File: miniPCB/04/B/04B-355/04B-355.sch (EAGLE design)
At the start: 45 parts

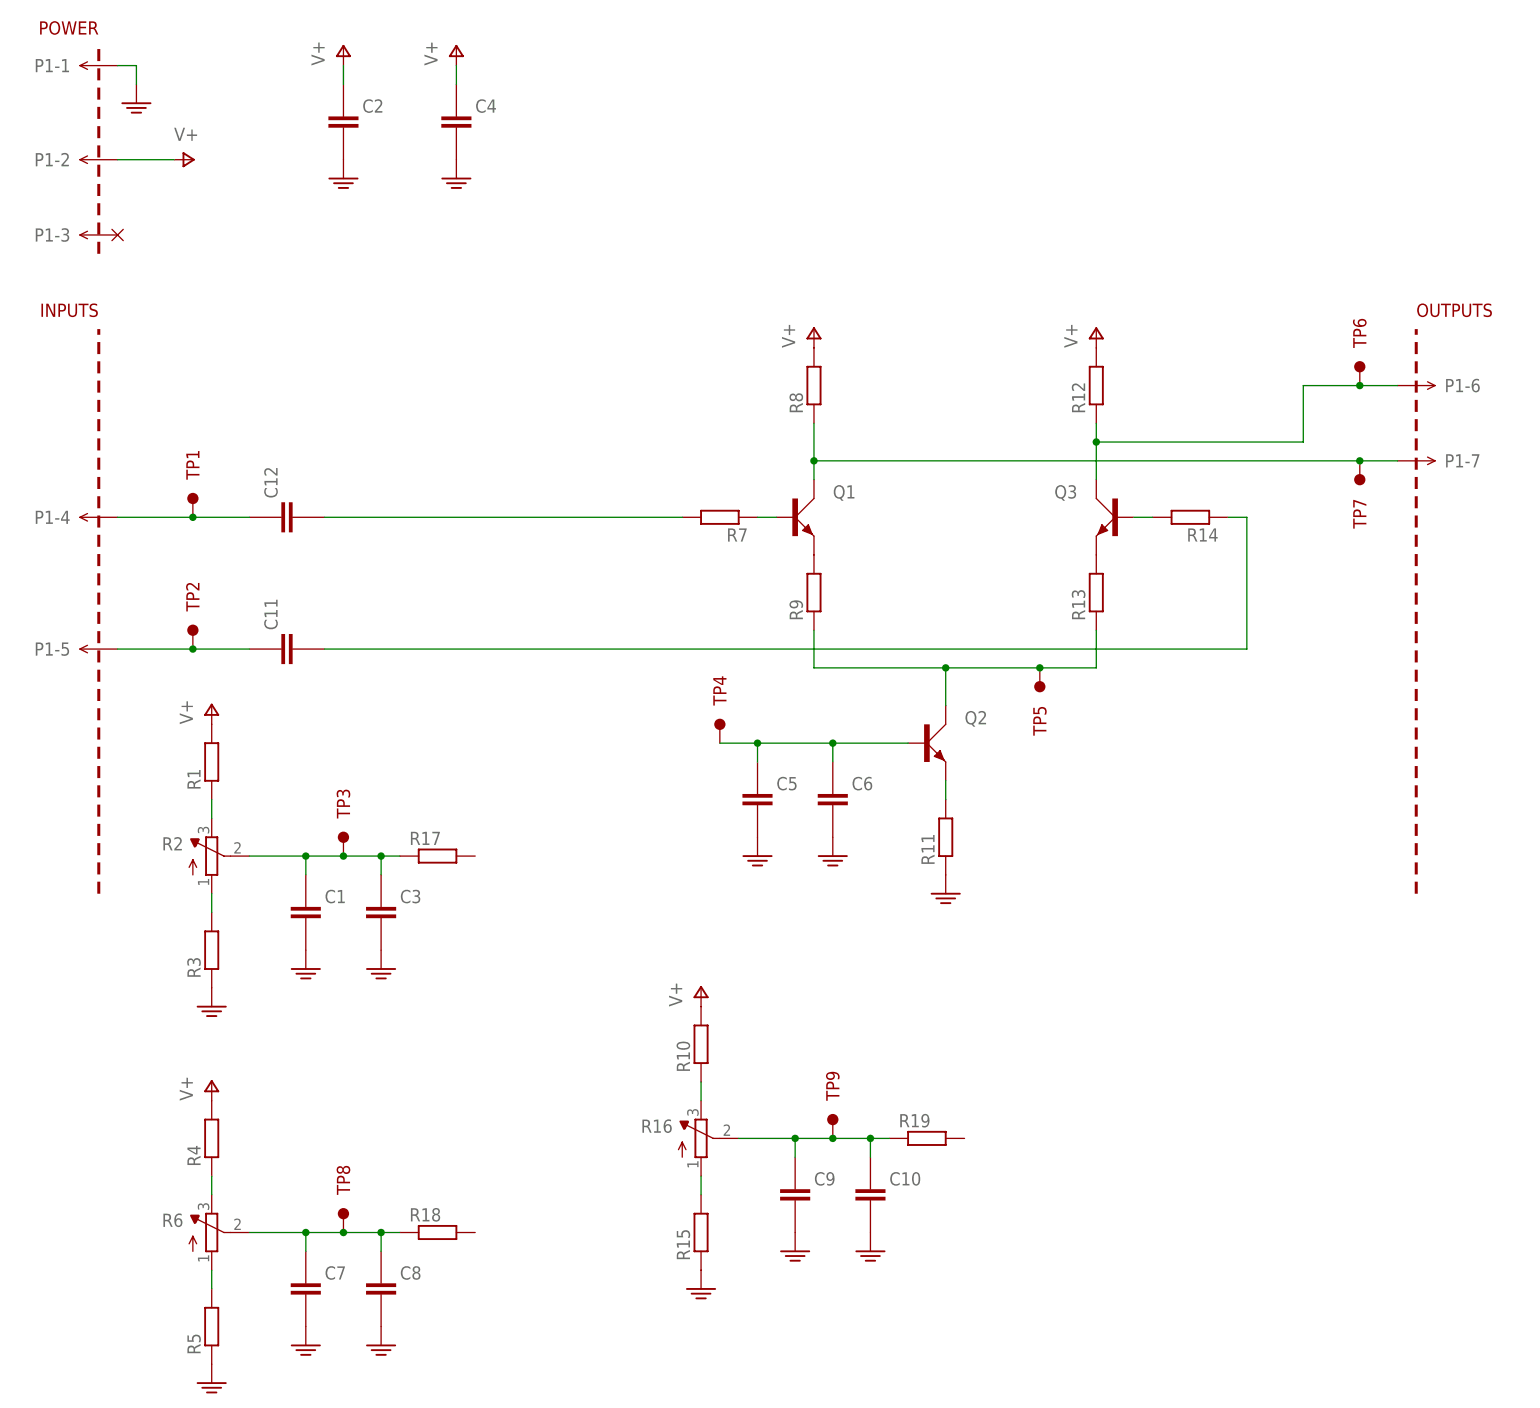
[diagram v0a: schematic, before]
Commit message: Attempting to fix my Git merge error.
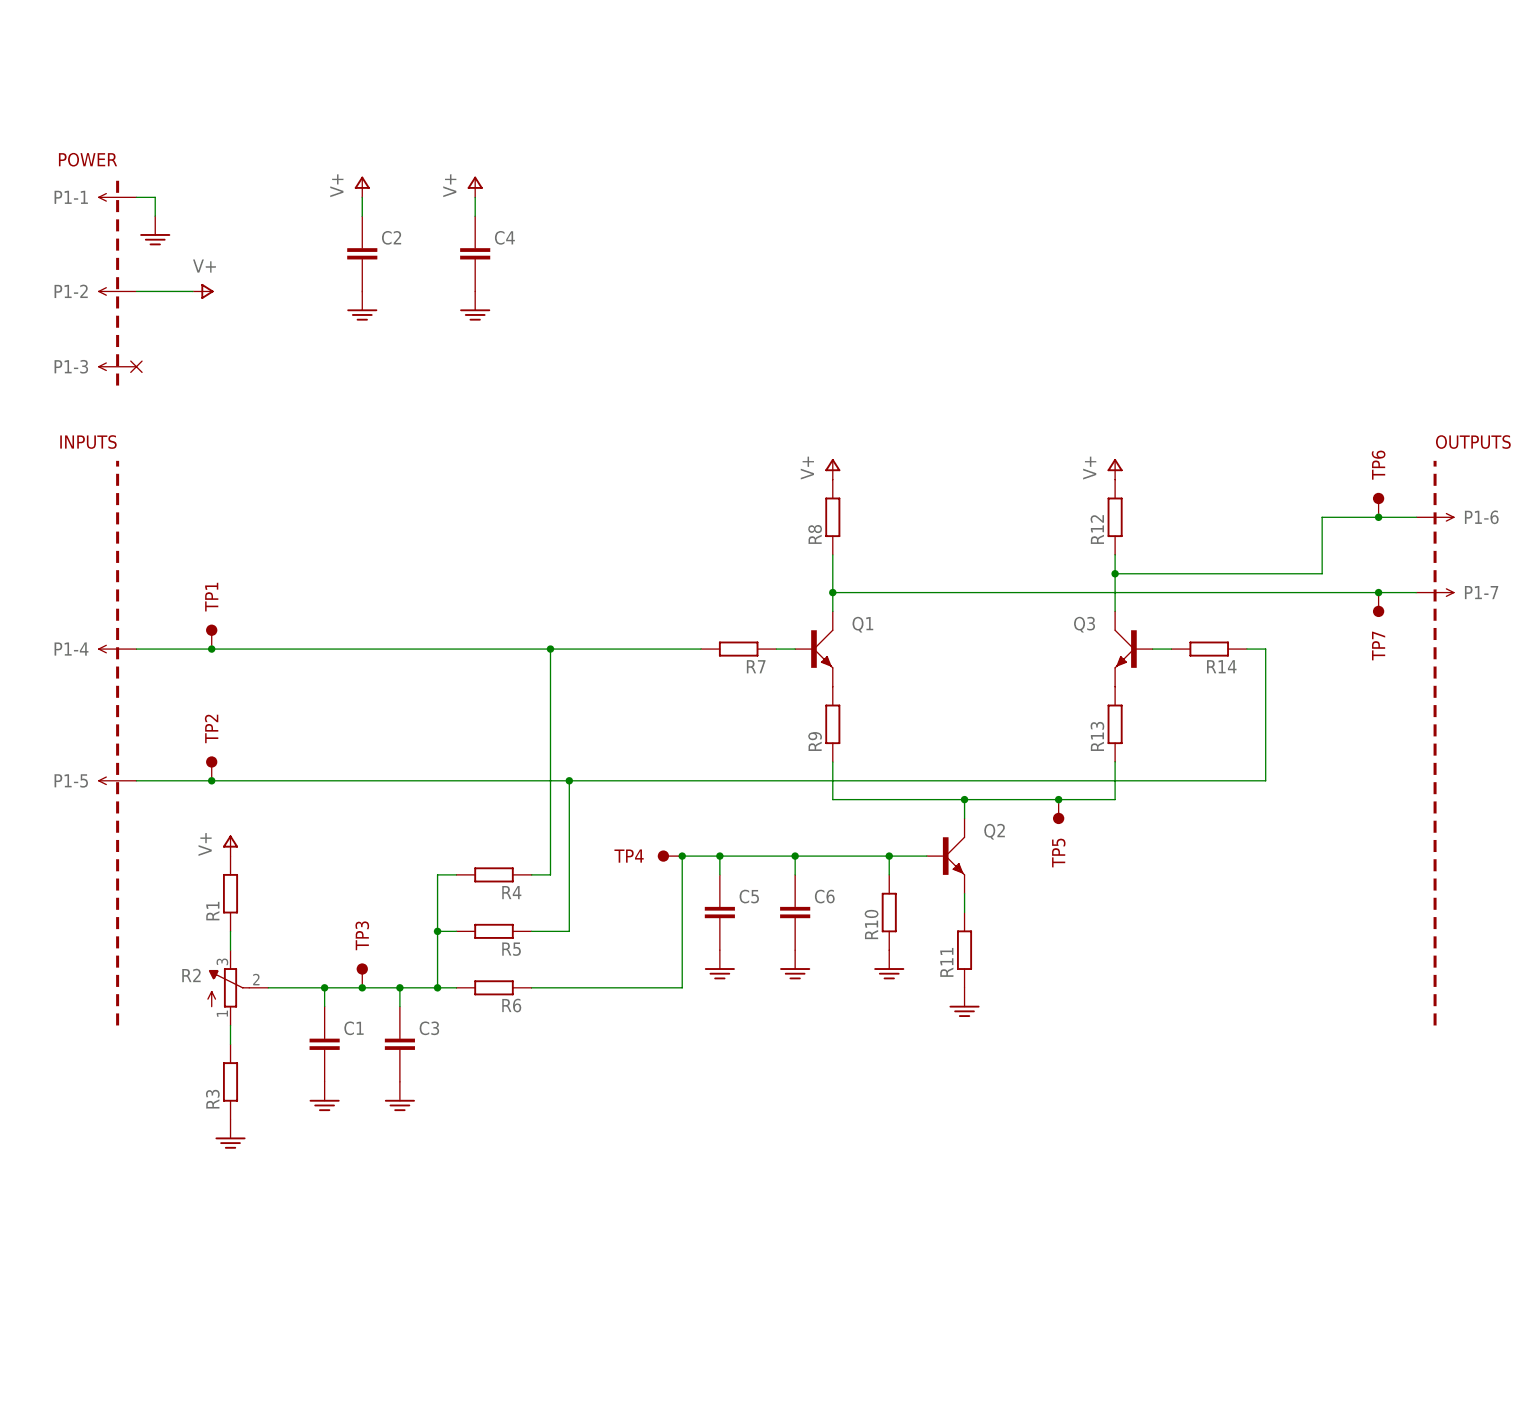
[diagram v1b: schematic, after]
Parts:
- removed C10, C8: (no value), minipcb:CAPACITOR_10
- removed C11, C12, C7, C9: (no value), minipcb:CAPACITORTHD
- removed R15, R17, R18, R19: (no value), minipcb:RESISTORTHD
- removed R16: (no value), minipcb:TRIMPOT0.100THD
- removed TP8, TP9: (no value), minipcb:TESTPOINTKE5000-SMTEXT
- R6: device minipcb:TRIMPOT0.100THD -> minipcb:RESISTORTHD
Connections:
- removed net N$15: R4.1, R6.E
- removed net N$16: R5.2, R6.A
- removed net N$17: C7.+, C8.+, R18.1, R6.S, TP8.1
- removed net N$18: R10.1, R16.E
- removed net N$19: R15.2, R16.A
- removed net N$20: C10.+, C9.+, R16.S, R19.1, TP9.1
- removed net N$21: C11.+, P1-5.1, TP2.1
- removed net N$22: C12.+, P1-4.1, TP1.1
- net GND: now also R10.1; no longer C10.-, C7.-, C8.-, C9.-, R15.1, R5.1
- net N$12: now also R10.2, R6.1
- net N$14: now also R4.2, R5.2, R6.2; no longer R17.1
- net N$8: now also P1-4.1, R4.1, TP1.1; no longer C12.-
- net N$9: now also P1-5.1, R5.1, TP2.1; no longer C11.-
- net V+: no longer R10.2, R4.2
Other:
- moved on the sheet: C1, C2, C3, C4, C5, C6, P1-1, P1-2, P1-3, P1-4, P1-5, P1-6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

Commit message: Attempting to fix my Git merge error.
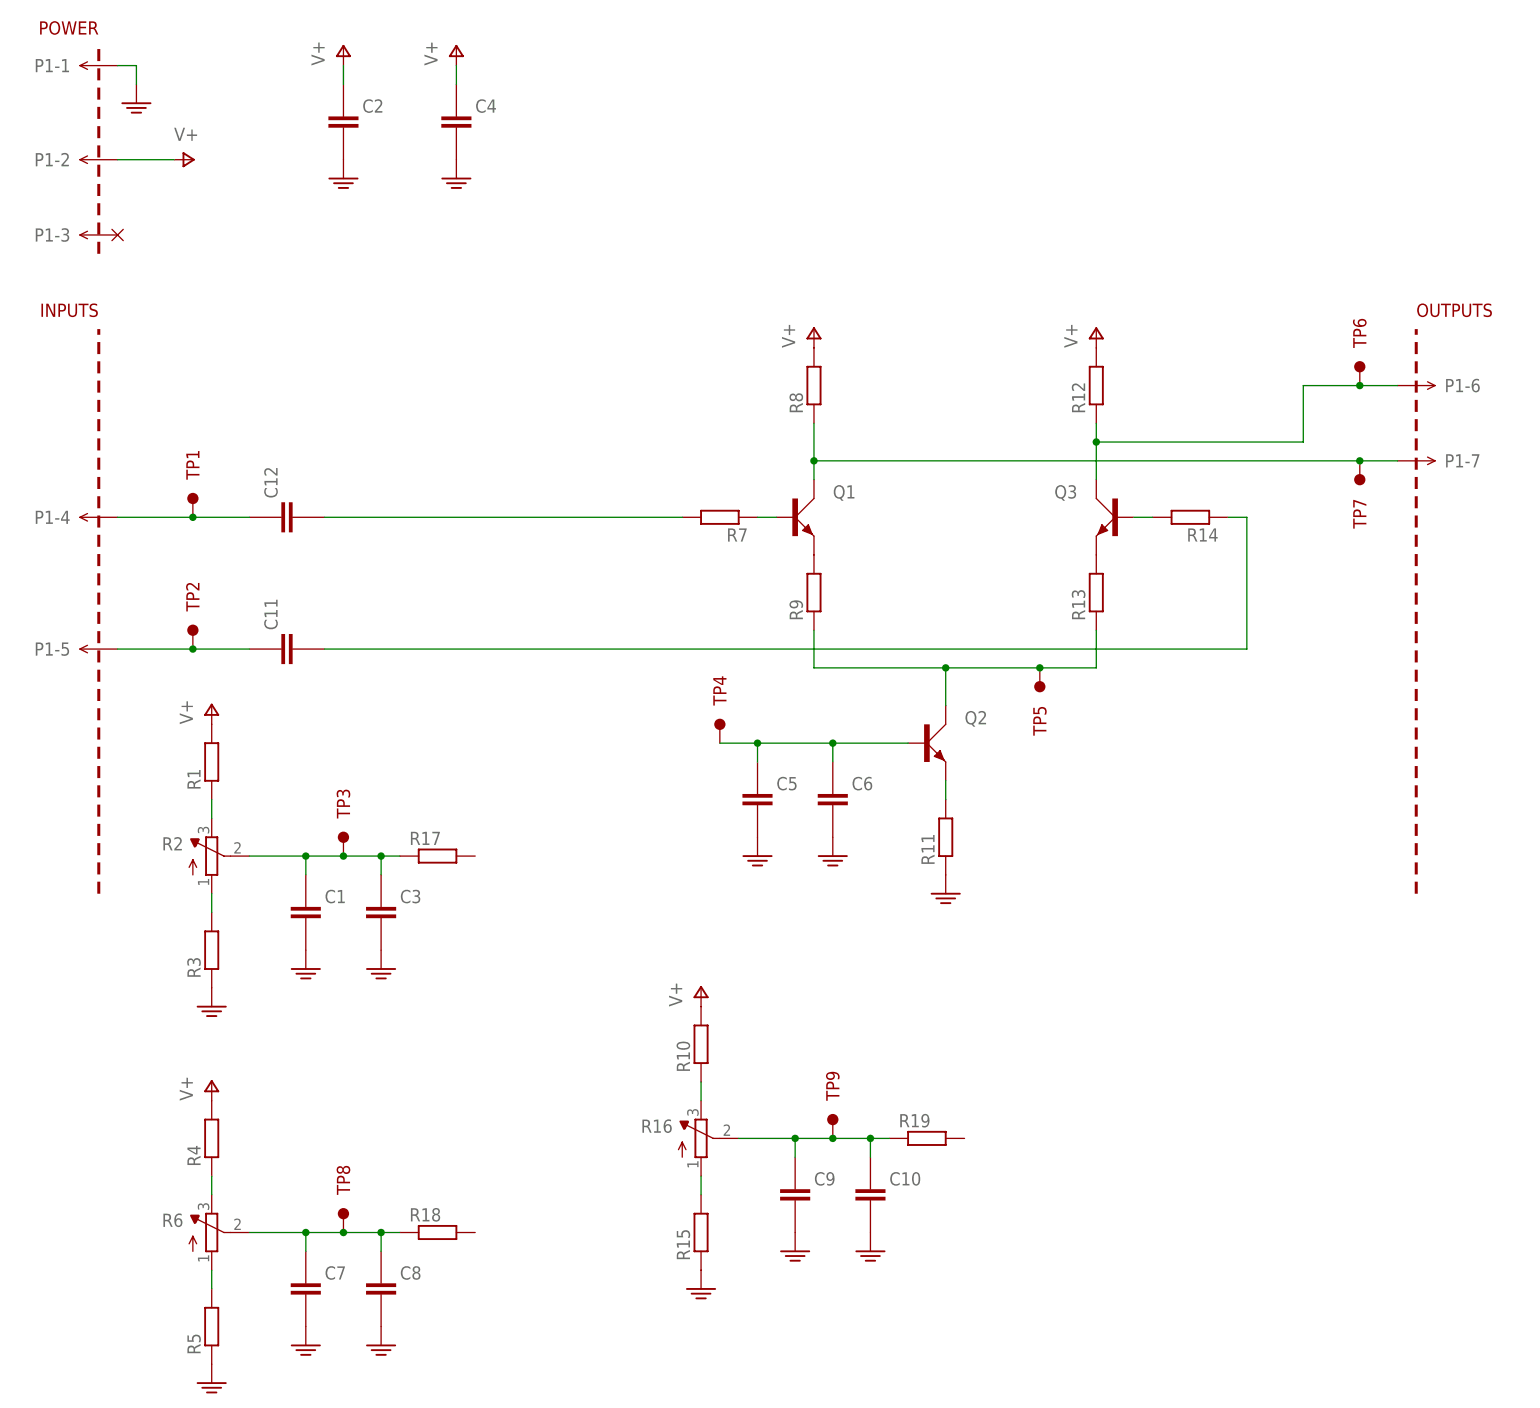
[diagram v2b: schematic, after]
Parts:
- added C10, C8: (no value), minipcb:CAPACITOR_10
- added C11, C12, C7, C9: (no value), minipcb:CAPACITORTHD
- added R15, R17, R18, R19: (no value), minipcb:RESISTORTHD
- added R16: (no value), minipcb:TRIMPOT0.100THD
- added TP8, TP9: (no value), minipcb:TESTPOINTKE5000-SMTEXT
- R6: device minipcb:RESISTORTHD -> minipcb:TRIMPOT0.100THD
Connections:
- new net N$15: R4.1, R6.E
- new net N$16: R5.2, R6.A
- new net N$17: C7.+, C8.+, R18.1, R6.S, TP8.1
- new net N$18: R10.1, R16.E
- new net N$19: R15.2, R16.A
- new net N$20: C10.+, C9.+, R16.S, R19.1, TP9.1
- new net N$21: C11.+, P1-5.1, TP2.1
- new net N$22: C12.+, P1-4.1, TP1.1
- net GND: now also C10.-, C7.-, C8.-, C9.-, R15.1, R5.1; no longer R10.1
- net N$12: no longer R10.2, R6.1
- net N$14: now also R17.1; no longer R4.2, R5.2, R6.2
- net N$8: now also C12.-; no longer P1-4.1, R4.1, TP1.1
- net N$9: now also C11.-; no longer P1-5.1, R5.1, TP2.1
- net V+: now also R10.2, R4.2
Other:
- moved on the sheet: C1, C2, C3, C4, C5, C6, P1-1, P1-2, P1-3, P1-4, P1-5, P1-6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
